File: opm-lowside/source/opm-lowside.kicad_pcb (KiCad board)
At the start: 2 copper layers, 58 x 40 mm, 83 parts, among them IC1 INA180A3IDBVR, IC2 INA180A3IDBVR, IC3 INA180A3IDBVR, IC4 QFN37_7X7_TRI, J1 Current Sensing, J2 SPI/Info, J3 VCC_IO, J4 PWMx6, J5 Temperature, Q1 HYG025N06LS1C2, Q2 HYG025N06LS1C2, Q3 HYG025N06LS1C2, Q4 HYG025N06LS1C2, Q5 HYG025N06LS1C2, Q6 HYG025N06LS1C2, U1 TerminalBlock_2_P5.08mm, U2 TerminalBlock_3_P5.08mm

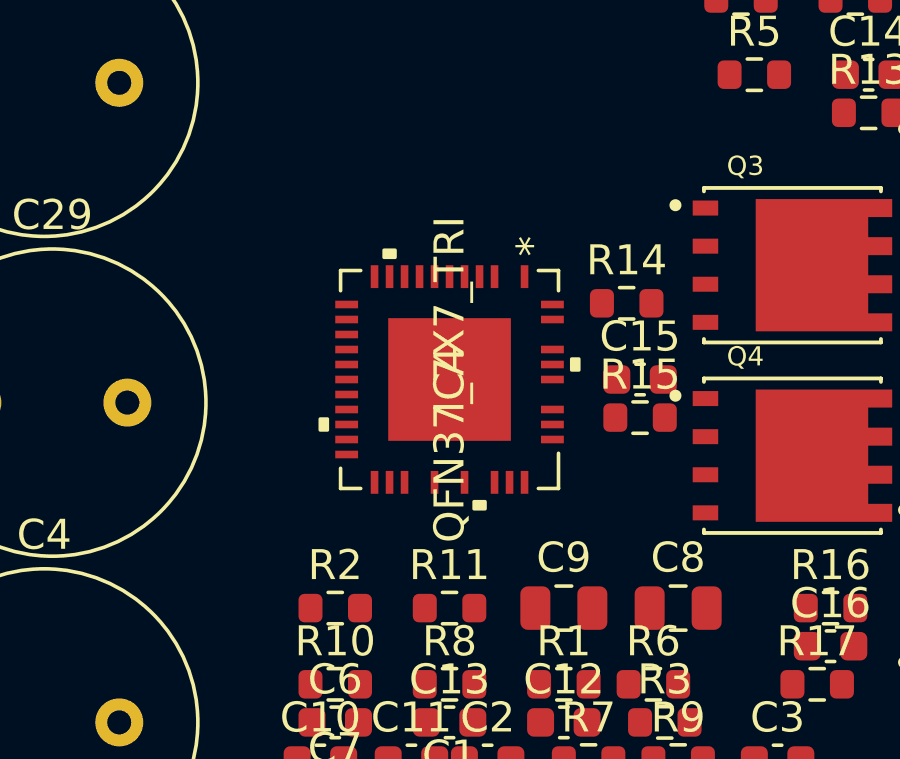
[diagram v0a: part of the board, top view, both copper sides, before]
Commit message: update parts
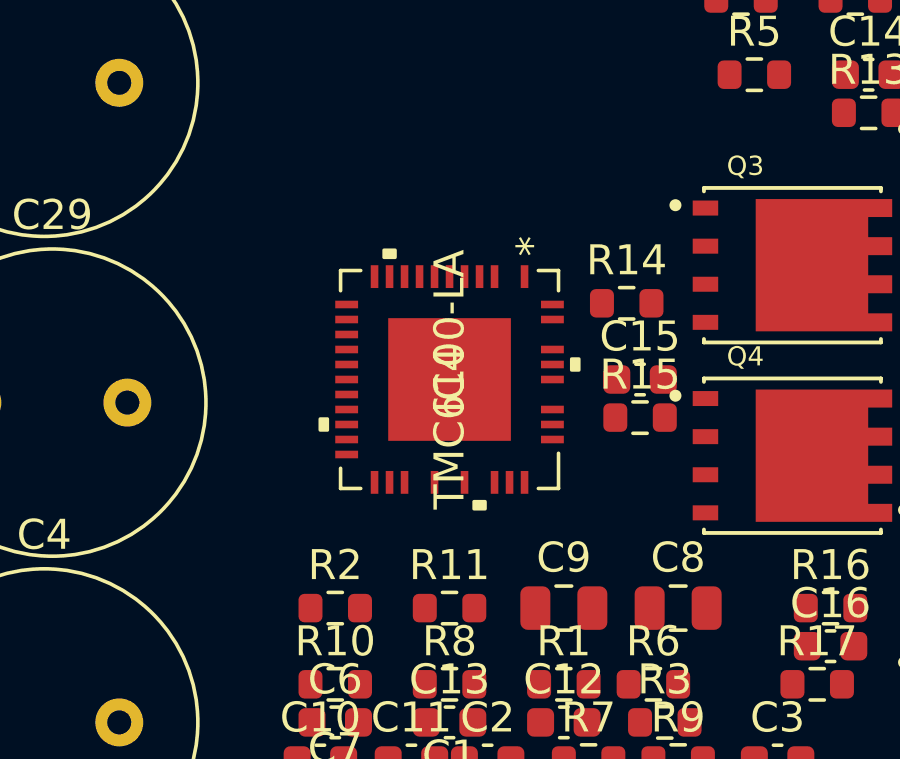
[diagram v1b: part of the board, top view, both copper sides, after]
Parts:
- C17: value 2,2μF/100V -> 2.2μF/100V
- IC4: value QFN37_7X7_TRI -> TMC6100-LA
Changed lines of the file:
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@@
       (effects (font (size 1 1) (thickness 0.15)))
     )
-    (fp_text value 2,2μF/100V (at 0 2.3 90) (layer F.Fab)
+    (fp_text value 2.2μF/100V (at 0 2.3 90) (layer F.Fab)
       (effects (font (size 1 1) (thickness 0.15)))
     )
@@
       (effects (font (size 1 1) (thickness 0.15)))
     )
-    (fp_text value QFN37_7X7_TRI (at 0 0 90) (layer F.SilkS)
-      (effects (font (size 1 1) (thickness 0.15)))
-    )
+    (fp_text value TMC6100-LA (at 0 0 90) (layer F.SilkS)
+      (effects (font (size 1 1) (thickness 0.15)))
+    )
